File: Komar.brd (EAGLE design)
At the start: 59.2 x 59.2 mm, 113 parts, among them CON10 PINHEAD_1X01-2, CON11 PINHEAD_1X01-2, CON12 PINHEAD_1X01-2, CON13 PINHEAD_1X01-2, CON14 PINHEAD_1X01-2, CON15 PINHEAD_1X01-2, CON2 PINHEAD_1X01-2, CON3 CON-4P-TABS-STRAIGHT, CON4 CON-4P-TABS-STRAIGHT, CON5 CON-4P-TABS-STRAIGHT, CON6 CON-4P-TABS-STRAIGHT, CON7 CON-4P-TABS-STRAIGHT, CON8 PINHEAD_1X04-2, CON9 PINHEAD_1X01-2, IC1 TPD3S014DBVR-SOT23-6, IC2 TPD3S014DBVR-SOT23-6, IC3 ATA6561-GBQW-N-HVSON8, IC4 ATA6561-GBQW-N-HVSON8, IC5 MCP9700AT-E/TTVAO-SOT23, IC6 11LC040T-E/TT, J1 105133-0011, Q1 FDMS86368-F085, Q10 FDMS86368-F085, Q11 FDMS86368-F085, Q12 FDMS86368-F085, Q2 FDMS86368-F085, Q3 FDMS86368-F085, Q4 FDMS86368-F085, Q5 FDMS86368-F085, Q6 FDMS86368-F085, Q7 FDMS86368-F085, Q8 FDMS86368-F085, Q9 FDMS86368-F085

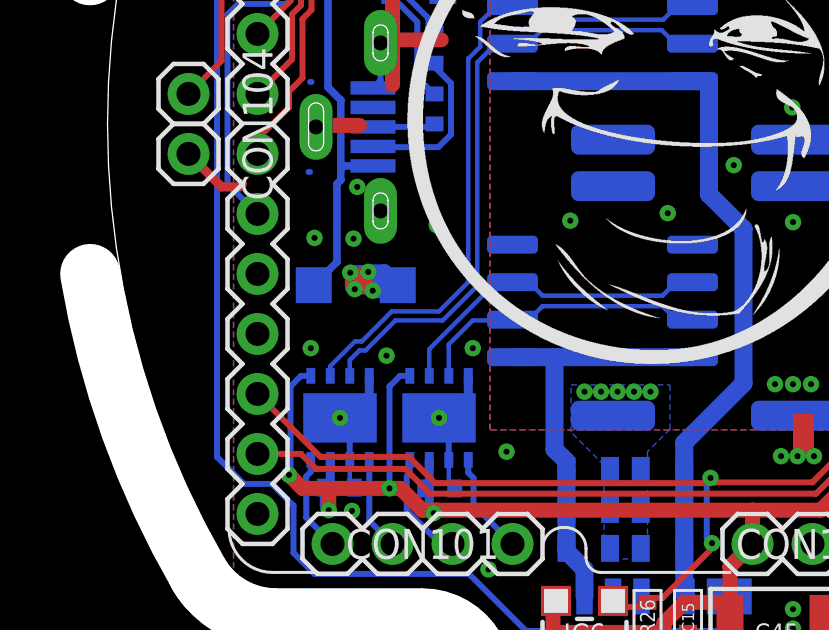
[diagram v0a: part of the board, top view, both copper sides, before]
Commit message: updated power via connection
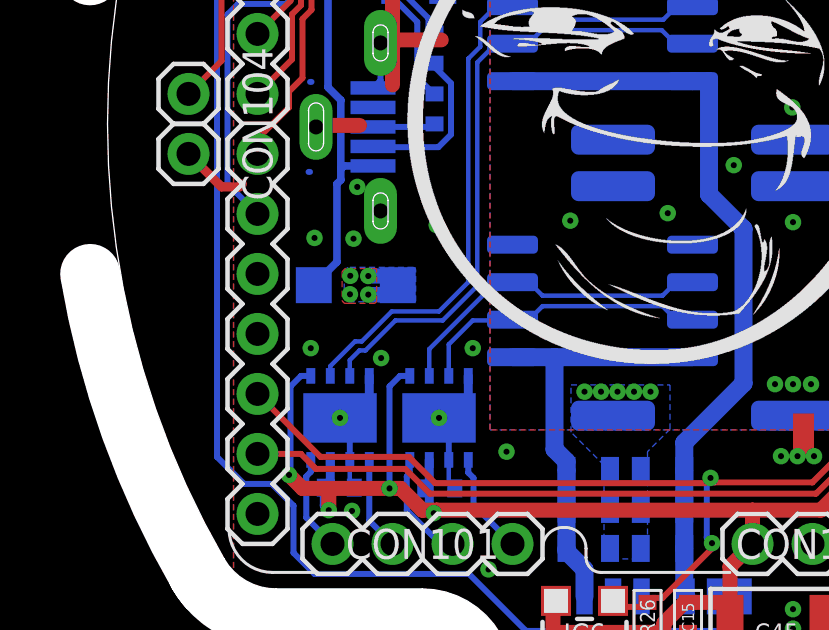
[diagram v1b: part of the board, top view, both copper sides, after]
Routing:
- net VDD_5V: track 169.4 -> 158.7 mm
- added copper zone on layer 1, net VDD_5V
- added copper zone on layer 15, net VDD_5V
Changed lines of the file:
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@@
 <setting verticaltext="up"/>
 </settings>
-<grid distance="0.1" unitdist="mm" unit="mm" style="lines" multiple="29" display="yes" altdistance="0.1" altunitdist="mm" altunit="mm"/>
+<grid distance="0.01" unitdist="mm" unit="mm" style="lines" multiple="29" display="yes" altdistance="0.1" altunitdist="mm" altunit="mm"/>
 <layers>
 <layer number="1" name="Top" color="4" fill="1" visible="yes" active="yes"/>
@@
 <wire x1="11.375" y1="17.8" x2="11.375" y2="18.875" width="0.2" layer="16"/>
 <wire x1="11.375" y1="18.875" x2="11.075" y2="19.175" width="0.2" layer="16"/>
-<via x="9.3" y="21.275" extent="1-16" drill="0.2" diameter="0.55"/>
+<via x="9.12" y="21.195" extent="1-16" drill="0.2" diameter="0.55"/>
 <via x="12.175" y="21.525" extent="1-16" drill="0.2" diameter="0.55"/>
 <via x="29.375" y="43.85" extent="1-16" drill="0.2" diameter="0.55"/>
@@
 <contactref element="LED2" pad="A"/>
 <contactref element="R27" pad="2"/>
-<via x="8.09126875" y="24.04126875" extent="1-16" drill="0.2" diameter="0.55"/>
-<via x="8.84126875" y="23.44126875" extent="1-16" drill="0.2" diameter="0.55"/>
-<via x="8.69126875" y="24.06626875" extent="1-16" drill="0.2" diameter="0.55"/>
+<via x="8.69126875" y="23.93126875" extent="1-16" drill="0.2" diameter="0.55"/>
+<via x="8.08126875" y="23.32126875" extent="1-16" drill="0.2" diameter="0.55"/>
+<via x="8.09126875" y="23.93626875" extent="1-16" drill="0.2" diameter="0.55"/>
 <contactref element="D7" pad="2"/>
 <contactref element="D7" pad="5"/>
@@
 <wire x1="17.1" y1="46.975" x2="17.1" y2="46.475" width="0.4" layer="1"/>
 <contactref element="MODULE2" pad="40"/>
-<via x="8.24126875" y="23.49126875" extent="1-16" drill="0.2" diameter="0.55"/>
-<wire x1="11.725" y1="20.74163125" x2="8.801321875" y2="23.5014" width="0.5" layer="15"/>
-<wire x1="8.801321875" y1="23.5014" x2="8.44126875" y2="23.84126875" width="0.5" layer="15"/>
+<via x="8.69126875" y="23.31126875" extent="1-16" drill="0.2" diameter="0.55"/>
 <wire x1="11.725" y1="18.45" x2="14.025" y2="16.15" width="0.5" layer="15"/>
 <wire x1="14.025" y1="16.15" x2="20.075" y2="16.15" width="0.5" layer="15"/>
 <wire x1="21.5" y1="15" x2="21.225" y2="15" width="0.5" layer="15"/>
 <wire x1="21.225" y1="15" x2="20.075" y2="16.15" width="0.5" layer="15"/>
-<wire x1="11.725" y1="20.74163125" x2="11.725" y2="18.45" width="0.5" layer="15"/>
+<wire x1="11.725" y1="18.45" x2="11.725" y2="20.74163125" width="0.5" layer="15"/>
 <contactref element="IC6" pad="2"/>
 <contactref element="C15" pad="2"/>
@@
 <wire x1="20.7" y1="13.05" x2="20.75" y2="13" width="0.5" layer="1"/>
 <wire x1="18" y1="12.05" x2="18.55" y2="12.05" width="0.5" layer="1"/>
-<wire x1="8.69126875" y1="24" x2="8.69126875" y2="23.611453125" width="0.2" layer="15"/>
-<wire x1="8.69126875" y1="23.611453125" x2="8.801321875" y2="23.5014" width="0.2" layer="15"/>
-<wire x1="8.84126875" y1="23.44126875" x2="8.69126875" y2="23.59126875" width="0.508" layer="15"/>
-<wire x1="8.69126875" y1="23.59126875" x2="8.69126875" y2="23.94126875" width="0.508" layer="15"/>
-<wire x1="8.24126875" y1="23.49126875" x2="8.791190625" y2="23.49126875" width="0.508" layer="15"/>
-<wire x1="8.791190625" y1="23.49126875" x2="8.801321875" y2="23.5014" width="0.508" layer="15"/>
-<wire x1="8.69126875" y1="24.06626875" x2="9.23373125" y2="24.06626875" width="0.508" layer="16"/>
-<wire x1="9.23373125" y1="24.06626875" x2="9.6" y2="23.7" width="0.508" layer="16"/>
-<wire x1="9.6" y1="23.7" x2="9.675" y2="23.625" width="0.508" layer="16"/>
-<wire x1="8.84126875" y1="23.44126875" x2="9.34126875" y2="23.44126875" width="0.508" layer="16"/>
-<wire x1="9.34126875" y1="23.44126875" x2="9.6" y2="23.7" width="0.508" layer="16"/>
-<wire x1="8.84126875" y1="23.44126875" x2="8.84126875" y2="23.91626875" width="0.508" layer="16"/>
-<wire x1="8.71626875" y1="24.04126875" x2="8.69126875" y2="24.06626875" width="0.508" layer="16"/>
-<wire x1="8.09126875" y1="24.04126875" x2="8.71626875" y2="24.04126875" width="0.508" layer="16"/>
-<wire x1="8.71626875" y1="24.04126875" x2="8.84126875" y2="23.91626875" width="0.508" layer="16"/>
-<wire x1="8.24126875" y1="23.49126875" x2="8.69126875" y2="23.94126875" width="0.508" layer="15"/>
-<wire x1="8.69126875" y1="23.94126875" x2="8.69126875" y2="24" width="0.508" layer="15"/>
-<wire x1="8.84126875" y1="23.44126875" x2="8.79126875" y2="23.49126875" width="0.3048" layer="1"/>
-<wire x1="8.69126875" y1="23.59126875" x2="8.79126875" y2="23.49126875" width="0.3048" layer="1"/>
-<wire x1="8.24126875" y1="23.49126875" x2="8.09126875" y2="23.64126875" width="0.3048" layer="1"/>
-<wire x1="8.09126875" y1="23.64126875" x2="8.09126875" y2="23.7" width="0.3048" layer="1"/>
-<wire x1="8.09126875" y1="23.7" x2="8.09126875" y2="24.04126875" width="0.3048" layer="1"/>
-<wire x1="8.24126875" y1="23.49126875" x2="8.79126875" y2="23.49126875" width="0.3048" layer="1"/>
-<wire x1="8.09126875" y1="24.04126875" x2="8.11626875" y2="24.06626875" width="0.3048" layer="1"/>
-<wire x1="8.11626875" y1="24.06626875" x2="8.69126875" y2="24.06626875" width="0.3048" layer="1"/>
-<wire x1="8.69126875" y1="24.06626875" x2="8.69126875" y2="23.9" width="0.3048" layer="1"/>
-<wire x1="8.69126875" y1="23.9" x2="8.69126875" y2="23.59126875" width="0.3048" layer="1"/>
-<wire x1="8.69126875" y1="24.06626875" x2="8.09126875" y2="23.7" width="0.2" layer="1"/>
-<wire x1="8.24126875" y1="23.49126875" x2="8.69126875" y2="23.9" width="0.2" layer="1"/>
-<wire x1="8.69126875" y1="24.06626875" x2="8.24126875" y2="23.49126875" width="0.2" layer="1"/>
-<wire x1="8.69126875" y1="24.06626875" x2="8.09126875" y2="24.04126875" width="0.2" layer="15"/>
-<wire x1="8.29126875" y1="23.44126875" x2="8.4" y2="23.44126875" width="0.254" layer="16"/>
-<wire x1="8.4" y1="23.44126875" x2="8.84126875" y2="23.44126875" width="0.254" layer="16"/>
-<wire x1="8.16626875" y1="23.96626875" x2="8.09126875" y2="24.04126875" width="0.508" layer="16"/>
-<wire x1="8.24126875" y1="23.49126875" x2="8.16626875" y2="23.56626875" width="0.508" layer="16"/>
-<wire x1="8.16626875" y1="23.56626875" x2="8.16626875" y2="23.96626875" width="0.508" layer="16"/>
-<wire x1="8.24126875" y1="23.49126875" x2="8.29126875" y2="23.44126875" width="0.15" layer="16"/>
-<wire x1="8.69126875" y1="24.06626875" x2="8.4" y2="23.44126875" width="0.15" layer="16"/>
-<wire x1="8.84126875" y1="23.44126875" x2="8.16626875" y2="23.96626875" width="0.15" layer="16"/>
+<polygon width="0.1524" layer="15">
+<vertex x="7.81" y="23.31"/>
+<vertex x="7.81" y="24.04"/>
+<vertex x="7.94" y="24.17"/>
+<vertex x="8.84" y="24.17"/>
+<vertex x="8.95" y="24.06"/>
+<vertex x="8.95" y="23.17"/>
+<vertex x="8.84" y="23.06"/>
+<vertex x="7.9" y="23.06"/>
+<vertex x="7.81" y="23.15"/>
+<vertex x="7.81" y="23.27"/>
+<vertex x="7.81" y="23.28"/>
+<vertex x="7.8" y="23.29"/>
+</polygon>
+<wire x1="11.725" y1="20.74163125" x2="9.1553625" y2="23.31126875" width="0.508" layer="15"/>
+<wire x1="9.1553625" y1="23.31126875" x2="9.1453625" y2="23.32126875" width="0.508" layer="15"/>
+<wire x1="9.1453625" y1="23.32126875" x2="8.08126875" y2="23.32126875" width="0.508" layer="15"/>
+<polygon width="0.2" layer="1">
+<vertex x="7.9" y="24.16"/>
+<vertex x="7.82" y="24.08"/>
+<vertex x="7.82" y="23.1"/>
+<vertex x="7.9" y="23.02"/>
+<vertex x="8.08" y="23.02"/>
+<vertex x="8.91" y="23.02"/>
+<vertex x="8.97" y="23.08"/>
+<vertex x="8.97" y="24.14"/>
+<vertex x="8.93" y="24.18"/>
+<vertex x="7.95" y="24.18"/>
+<vertex x="7.93" y="24.18"/>
+</polygon>
+<wire x1="8.69126875" y1="23.31126875" x2="9.1553625" y2="23.31126875" width="0.508" layer="15"/>
+<polygon width="0.15" layer="16">
+<vertex x="7.89" y="24"/>
+<vertex x="7.89" y="23.21"/>
+<vertex x="7.93" y="23.17"/>
+<vertex x="8.03" y="23.07"/>
+<vertex x="8.04" y="23.07"/>
+<vertex x="10.25" y="23.07"/>
+<vertex x="10.27" y="23.09"/>
+<vertex x="10.27" y="24.15"/>
+<vertex x="10.2" y="24.22"/>
+<vertex x="8.01" y="24.22"/>
+<vertex x="7.91" y="24.12"/>
+<vertex x="7.89" y="24.1"/>
+<vertex x="7.89" y="24.02"/>
+</polygon>
+<wire x1="8.69126875" y1="23.93126875" x2="9.36873125" y2="23.93126875" width="0.508" layer="16"/>
+<wire x1="9.36873125" y1="23.93126875" x2="9.675" y2="23.625" width="0.508" layer="16"/>
+<wire x1="8.69126875" y1="23.31126875" x2="9.36126875" y2="23.31126875" width="0.508" layer="16"/>
+<wire x1="9.36126875" y1="23.31126875" x2="9.675" y2="23.625" width="0.508" layer="16"/>
 </signal>
 <signal name="CAN1_VDD">
